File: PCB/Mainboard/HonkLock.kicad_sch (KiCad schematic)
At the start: 10 parts, among them J1 Conn_01x03_Pin, J5 Conn_01x02_Pin, U2 ESP32-S3-SUPERMINI

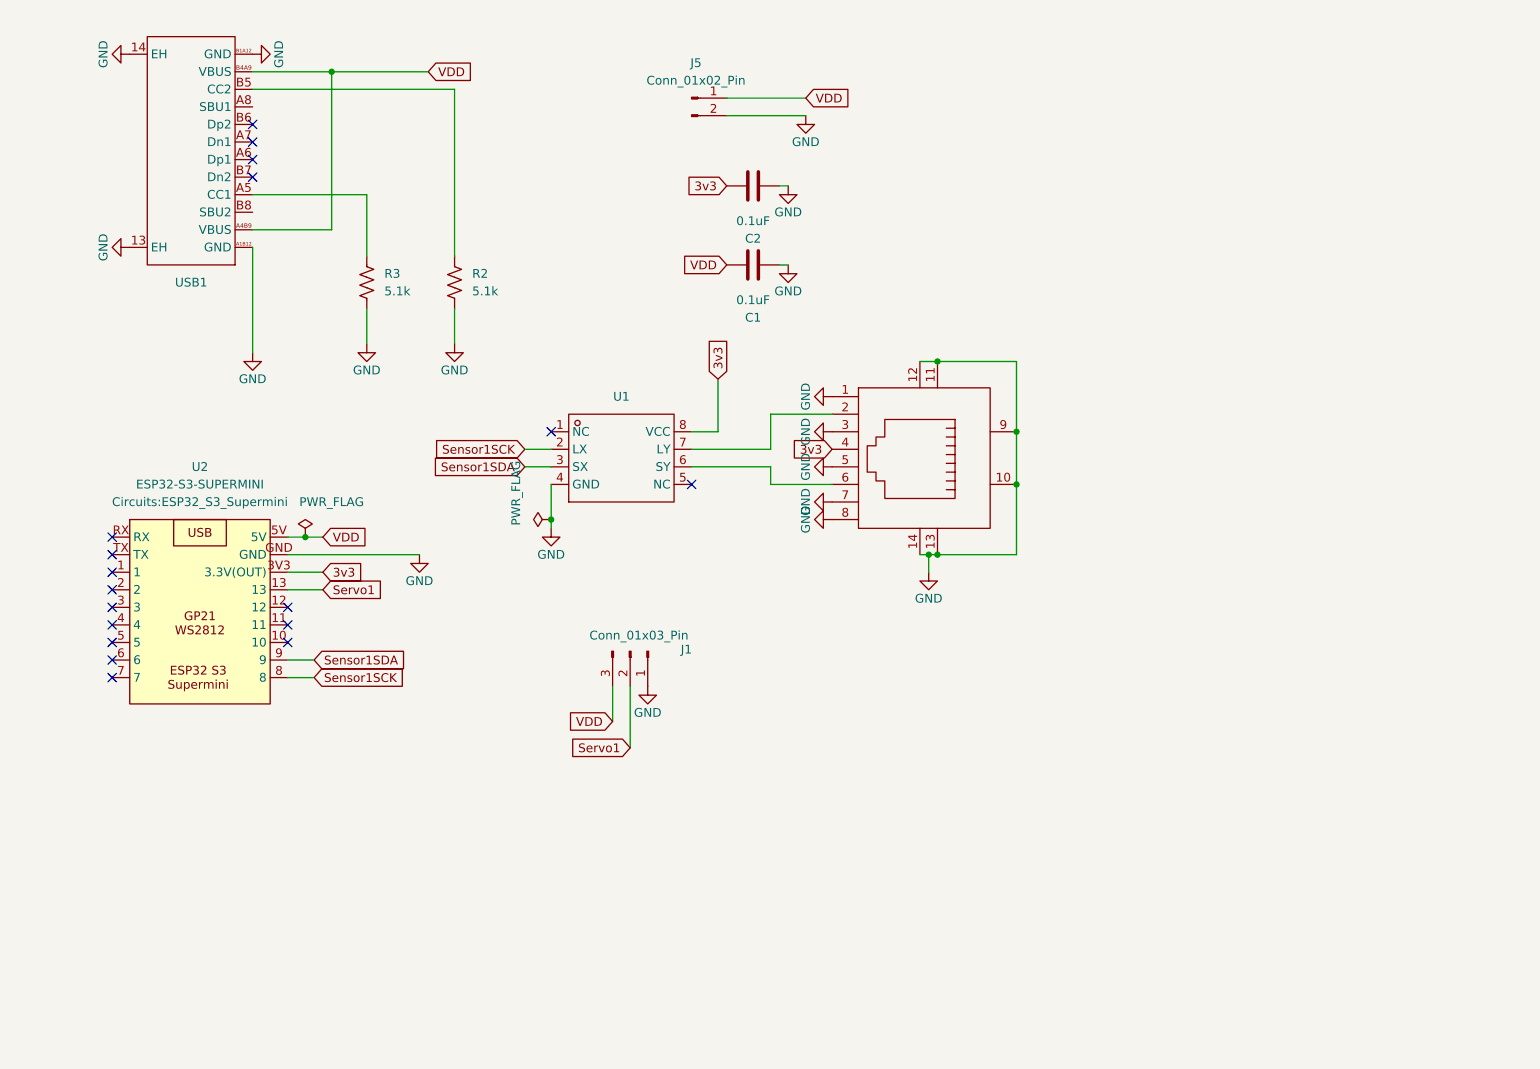
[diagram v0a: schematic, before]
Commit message: Mainboard ready for mfg
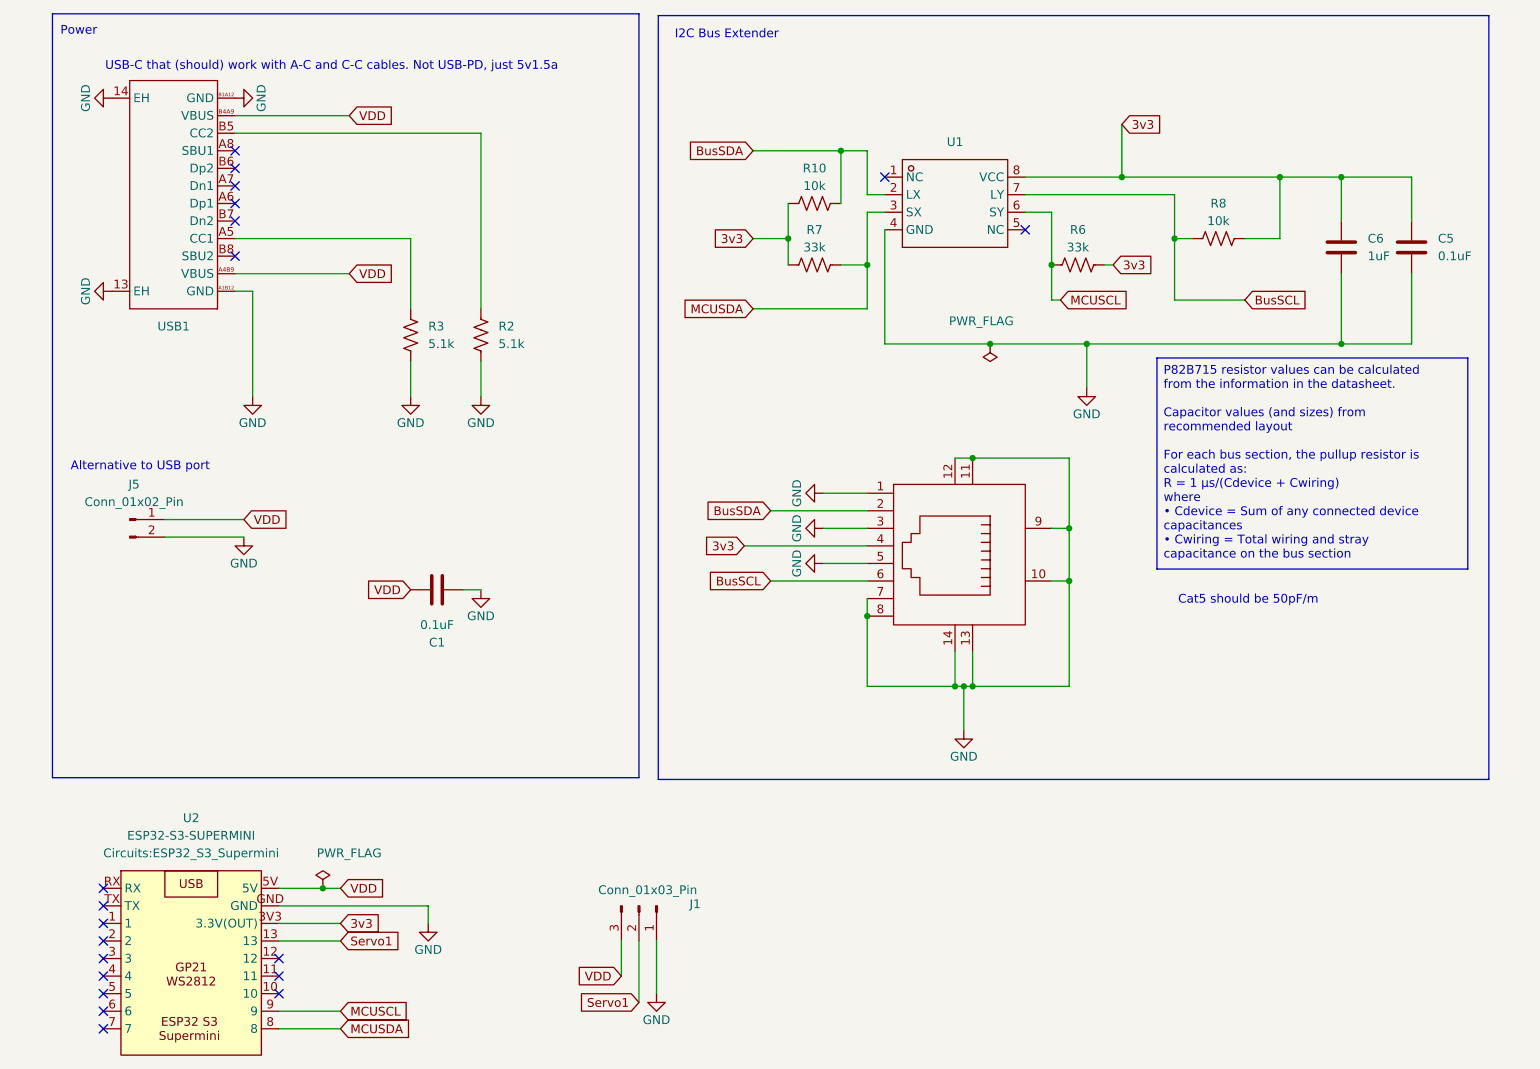
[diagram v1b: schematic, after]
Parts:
- removed C2: 0.1uF, Capacitor_SMD:C_1206_3216Metric, symbol Device:C
- added C5: 0.1uF, Capacitor_SMD:C_0805_2012Metric, symbol Device:C
- added C6: 1uF, Capacitor_SMD:C_0805_2012Metric, symbol Device:C
- added R10, R8: 10k, Resistor_SMD:R_0805_2012Metric, symbol PCM_SparkFun-Resistor:R
- added R6, R7: 33k, Resistor_SMD:R_0805_2012Metric, symbol PCM_SparkFun-Resistor:R
- C1: footprint Capacitor_SMD:C_1206_3216Metric -> Capacitor_SMD:C_0805_2012Metric
- R2, R3: footprint Resistor_SMD:R_1206_3216Metric -> Resistor_SMD:R_0805_2012Metric
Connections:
- net 3v3: now also C5.1, C6.1, R10.1, R6.2, R7.1, R8.2
- net GND: now also C5.2, C6.2
- net BusSCL: now reaches RJ1.6
- net BusSCL: now also U1.7 (LY), R8.1; no longer U1.6 (SY)
- net BusSDA: now reaches RJ1.2
- net BusSDA: now also U1.2 (LX), R10.2; no longer U1.7 (LY)
- net Sensor1SCK renamed MCUSDA
- net MCUSDA: now also U1.3 (SX), R7.2; no longer U1.2 (LX)
- net Sensor1SDA renamed MCUSCL
- net MCUSCL: now also U1.6 (SY), R6.1; no longer U1.3 (SX)
- no-connect marks 18 -> 20
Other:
- note added: "Alternative to USB port"
- note added: "Cat5 should be 50pF/m"
- note added: "I2C Bus Extender"
- note added: "Power"
- note added: "USB-C that (should) work with A-C and C-C cables. Not USB-PD, just 5v1.5a"
- company: (none) -> tmuWolverine
- title: (none) -> HonkLock
- moved on the sheet: C1, J1, J5, R2, R3, U1, U2, USB1
